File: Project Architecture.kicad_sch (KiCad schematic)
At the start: 0 parts

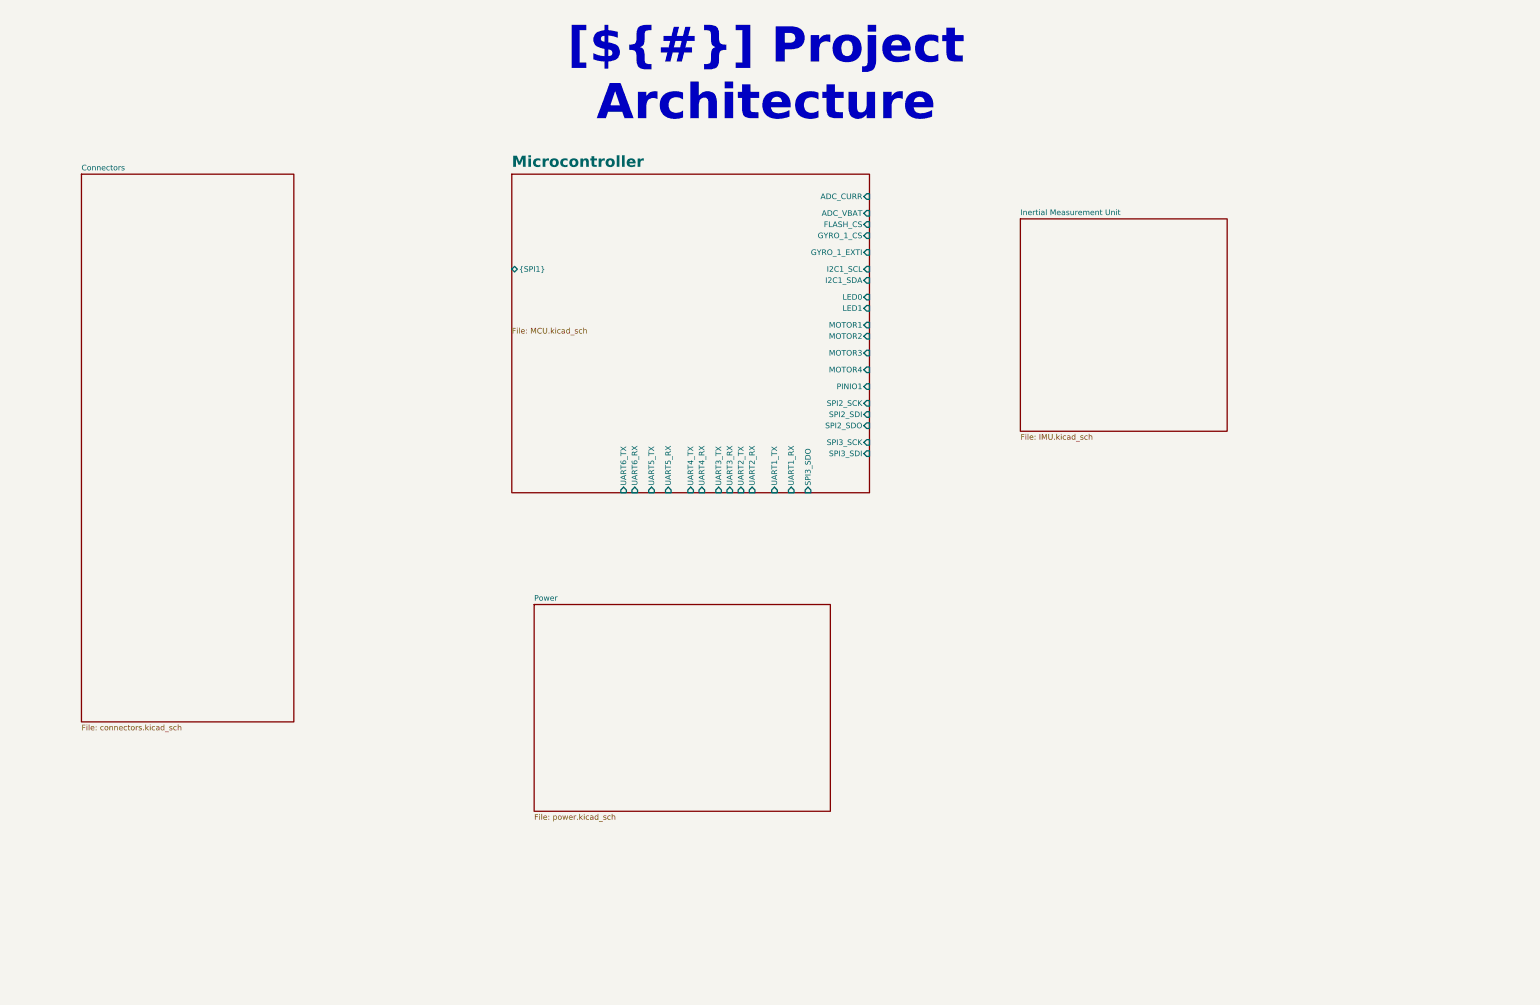
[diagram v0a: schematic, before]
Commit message: Finished system overview
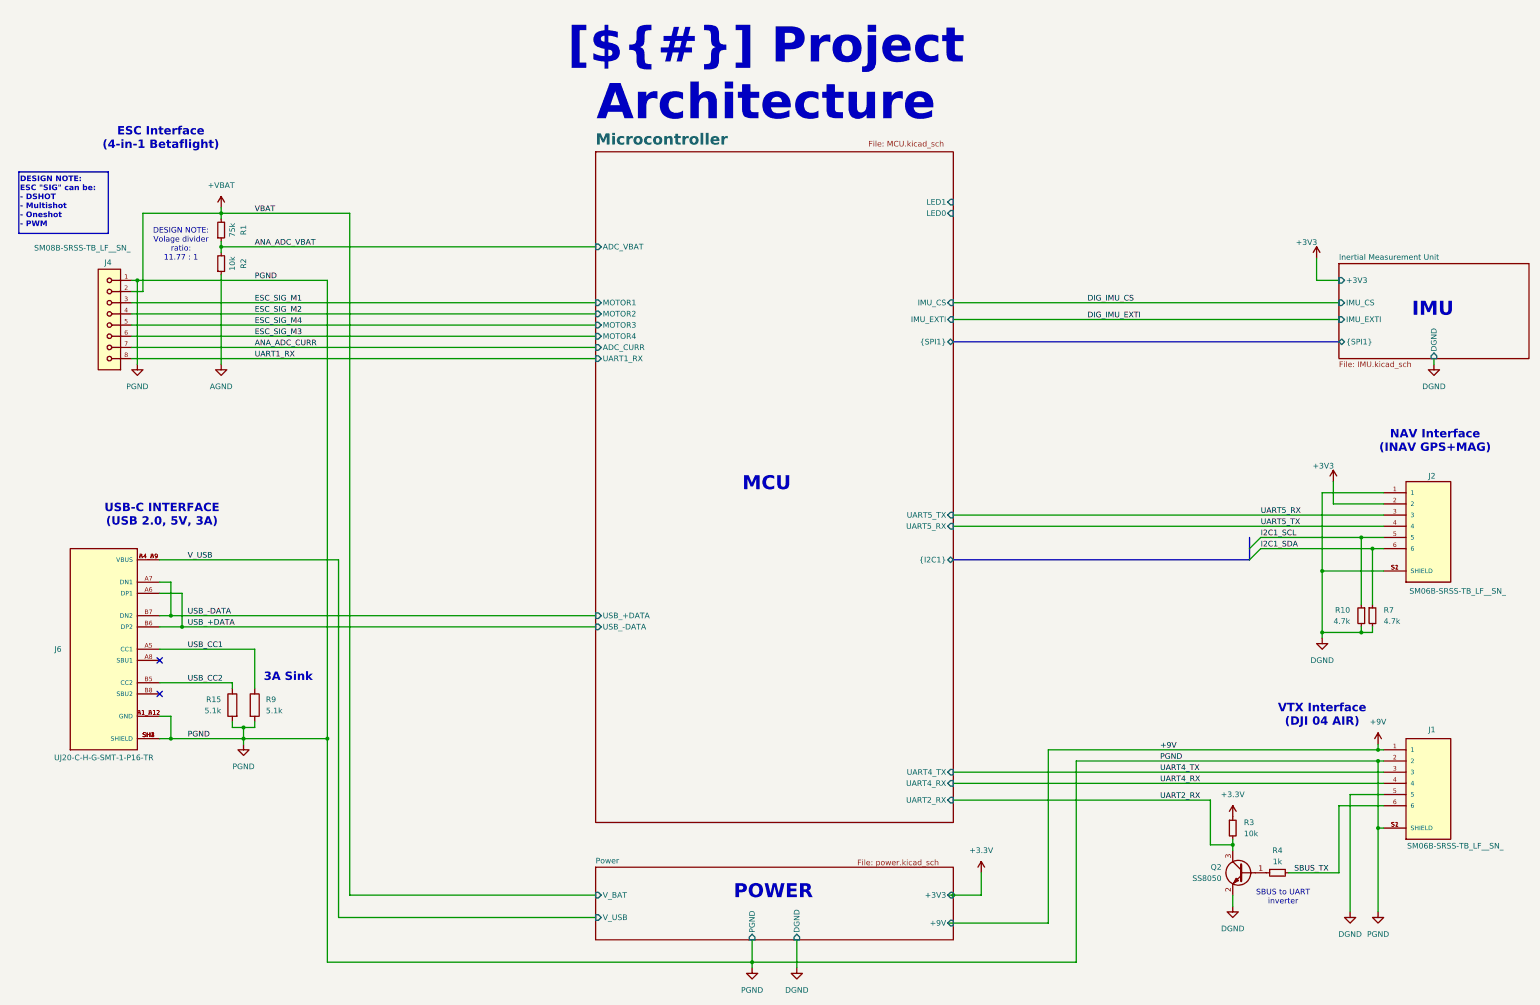
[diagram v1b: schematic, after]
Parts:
- added J1, J2: SM06B-SRSS-TB_LF__SN_, KSE_connector:JST_SM06B-SRSS-TB_LF__SN_, symbol KSE_connectors:SM06B-SRSS-TB_LF__SN_
- added J4: SM08B-SRSS-TB_LF__SN_, KSE_connector:JST_SM08B-SRSS-TB_LF__SN_, symbol KSE_connectors:SM08B-SRSS-TB_LF__SN_
- added J6: UJ20-C-H-G-SMT-1-P16-TR, KSE_connector:SAMESKY_UJ20-C-H-G-SMT-1-P16-TR, symbol KSE_connectors:UJ20-C-H-G-SMT-1-P16-TR
- added Q2: SS8050, Package_TO_SOT_SMD:SOT-23, symbol Transistor_BJT:SS8050
- added R1: 75k, Resistor_SMD:R_0603_1608Metric_Pad0.98x0.95mm_HandSolder, symbol Device:R_Small
- added R10, R7: 4.7k, Resistor_SMD:R_0603_1608Metric_Pad0.98x0.95mm_HandSolder, symbol Device:R_Small
- added R15, R9: 5.1k, Resistor_SMD:R_0805_2012Metric_Pad1.20x1.40mm_HandSolder, symbol Device:R
- added R2, R3: 10k, Resistor_SMD:R_0603_1608Metric_Pad0.98x0.95mm_HandSolder, symbol Device:R_Small
- added R4: 1k, Resistor_SMD:R_0603_1608Metric_Pad0.98x0.95mm_HandSolder, symbol Device:R_Small
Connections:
- new net: Q2.1 (B), R4.1
- new net +3.3V: R3.1
- new net +3V3: J2.2
- new net +9V: J1.1
- new net +VBAT: J4.2, R1.2
- new net AGND: R2.1
- new net ANA_ADC_CURR: J4.7
- new net ANA_ADC_VBAT: R1.1, R2.2
- new net DGND: J1.5, J2.1, J2.S1 (SHIELD), J2.S2 (SHIELD), Q2.2 (E), R10.2, R7.2
- new net ESC_SIG_M1: J4.3
- new net ESC_SIG_M2: J4.4
- new net ESC_SIG_M3: J4.6
- new net ESC_SIG_M4: J4.5
- new net I2C1_SCL: J2.5, R10.1
- new net I2C1_SDA: J2.6, R7.1
- new net PGND: J1.2, J1.S1 (SHIELD), J1.S2 (SHIELD), J4.1, J6.A1_B12 (GND), J6.B1_A12 (GND), J6.SH1 (SHIELD), J6.SH2 (SHIELD), J6.SH3 (SHIELD), J6.SH4 (SHIELD), R15.2, R9.2
- new net SBUS_TX: J1.6, R4.2
- new net UART1_RX: J4.8
- new net UART2_RX: Q2.3 (C), R3.2
- new net UART4_RX: J1.4
- new net UART4_TX: J1.3
- new net UART5_RX: J2.3
- new net UART5_TX: J2.4
- new net USB_+DATA: J6.A6 (DP1), J6.B6 (DP2)
- new net USB_-DATA: J6.A7 (DN1), J6.B7 (DN2)
- new net USB_CC1: J6.A5 (CC1), R9.1
- new net USB_CC2: J6.B5 (CC2), R15.1
- new net V_USB: J6.A4_B9 (VBUS), J6.B4_A9 (VBUS)
- no-connect marks 0 -> 2
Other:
- removed sheet Connectors
- sheet Inertial Measurement Unit ports: added +3V3, DGND, IMU_CS, IMU_EXTI, {SPI1}; removed none
- sheet Microcontroller ports: added IMU_CS, IMU_EXTI, USB_+DATA, USB_-DATA, {I2C1}; removed FLASH_CS, GYRO_1_CS, GYRO_1_EXTI, I2C1_SCL, I2C1_SDA, PINIO1, SPI2_SCK, SPI2_SDI, SPI2_SDO, SPI3_SCK, SPI3_SDI, SPI3_SDO, UART1_TX, UART2_TX, UART3_RX, UART3_TX, UART6_RX, UART6_TX
- sheet Power ports: added +3V3, +9V, DGND, PGND, V_BAT, V_USB; removed none
- note added: "3A Sink"
- note added: "DESIGN NOTE: ESC "SIG" can be: - DSHOT - Multishot - Oneshot - PWM"
- note added: "DESIGN NOTE: Volage divider ratio: 11.77 : 1"
- note added: "ESC Interface (4-in-1 Betaflight)"
- note added: "IMU"
- note added: "MCU"
- note added: "NAV Interface (INAV GPS+MAG)"
- note added: "POWER"
- note added: "SBUS to UART inverter"
- note added: "USB-C INTERFACE (USB 2.0, 5V, 3A)"
- note added: "VTX Interface (DJI 04 AIR)"
